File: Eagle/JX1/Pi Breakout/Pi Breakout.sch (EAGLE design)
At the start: 3 parts, among them J1 RASPBERRYPI-40-PIN-GPIO_PTH_N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, J2 RASPBERRYPI-40-PIN-GPIO_PTH_N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

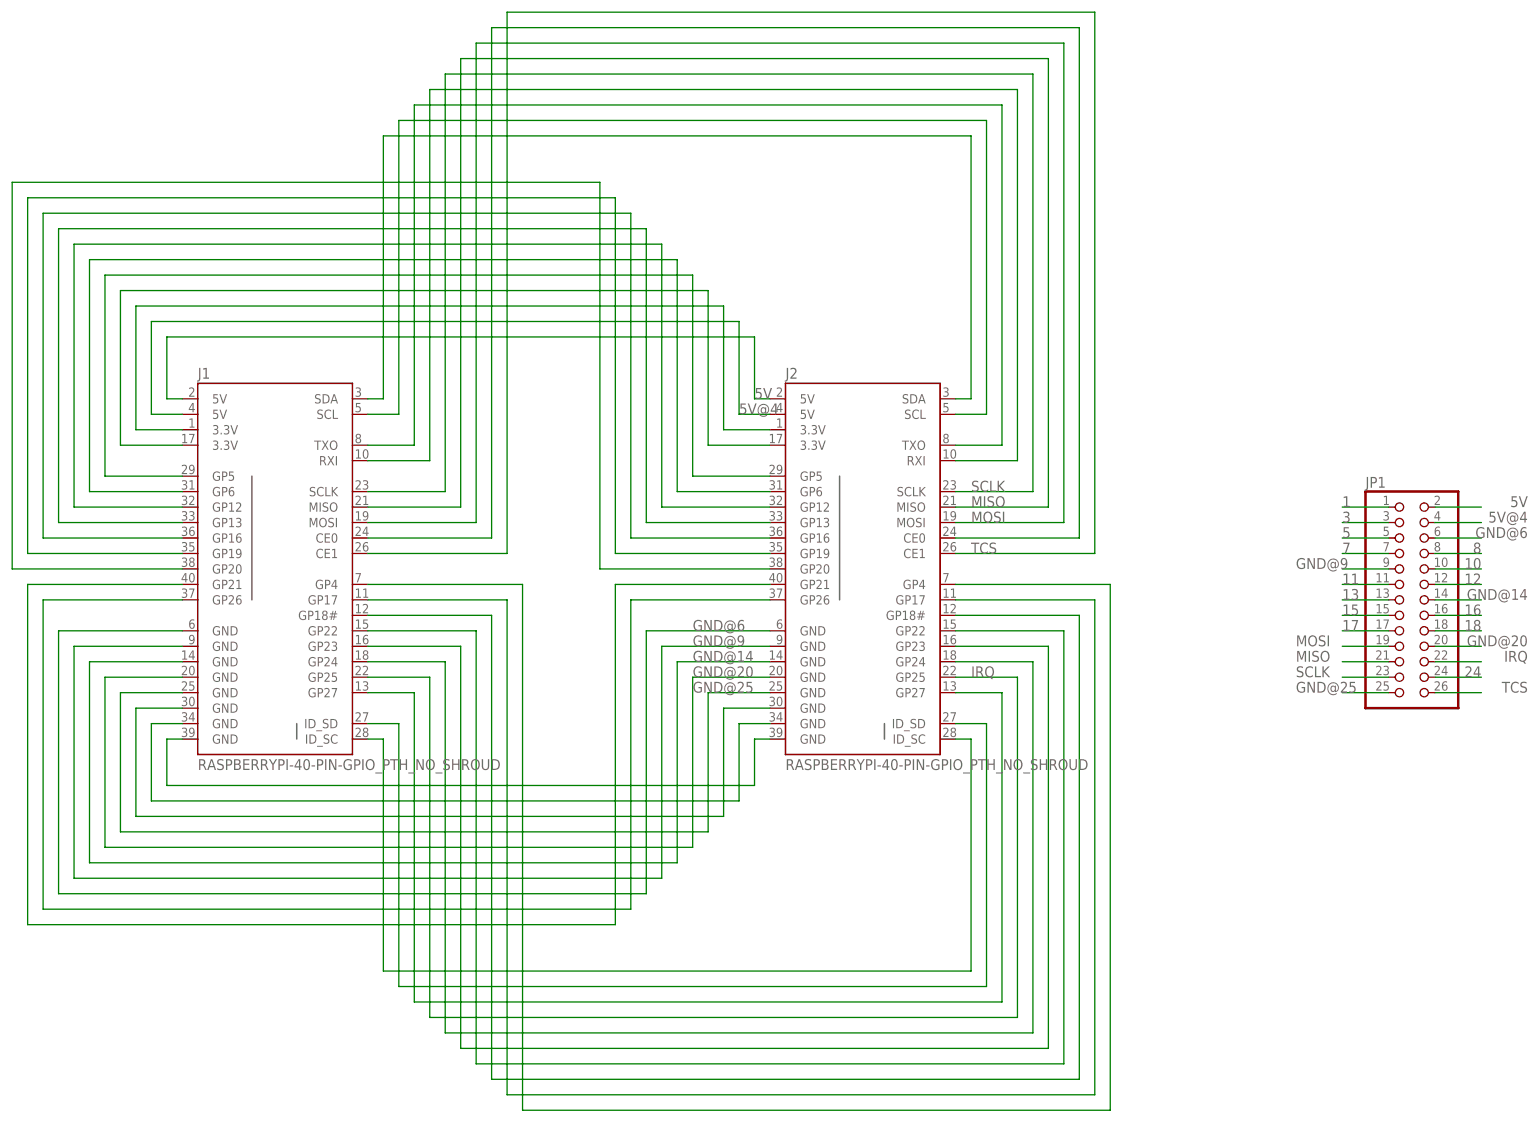
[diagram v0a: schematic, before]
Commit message: More board Changes
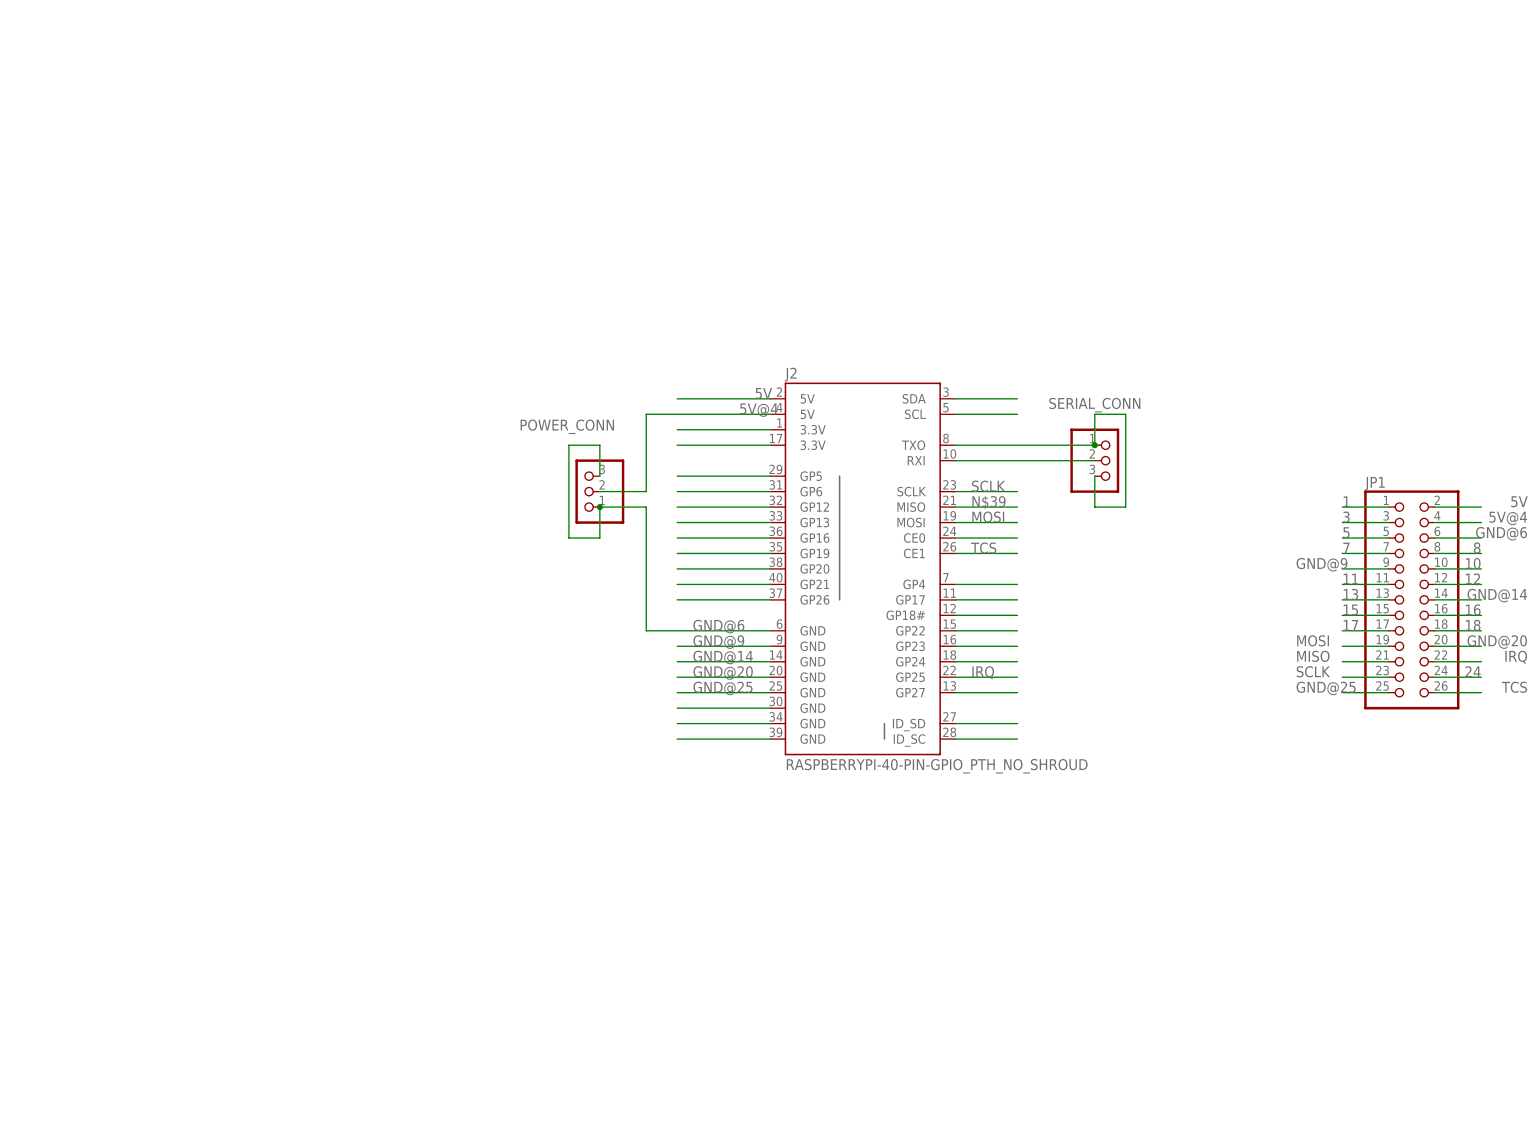
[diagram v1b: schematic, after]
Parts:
- removed J1: RASPBERRYPI-40-PIN-GPIO_PTH_NO_SHROUD, SparkFun-Connectors:RASPBERRYPI-40-PIN-GPIO_PTH_NO_SHROUD
- added POWER_CONN, SERIAL_CONN: (no value), pinhead:PINHD-1X3
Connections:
- removed net N$28: J1.SDA, J2.SDA
- removed net N$30: J1.RXI, J2.RXI
- removed net N$31: J1.TXO, J2.TXO
- removed net N$35: J1.CE0, J2.CE0
- new net N$1: J2.TXO, SERIAL_CONN.1, SERIAL_CONN.3
- new net N$25: J2.SDA
- new net N$32: J2.RXI, SERIAL_CONN.2
- new net N$33: J2.CE0
- new net N$39: J2.MISO
- net 5V: no longer J1.5V@2
- net 5V@4: now also POWER_CONN.2; no longer J1.5V@4
- net GND@14: no longer J1.GND@14
- net GND@20: no longer J1.GND@20
- net GND@25: no longer J1.GND@25
- net GND@6: now also POWER_CONN.1, POWER_CONN.3; no longer J1.GND@6
- net GND@9: no longer J1.GND@9
- net GP22: no longer J1.GP22
- net IRQ: no longer J1.GP25
- net MISO: no longer J1.MISO, J2.MISO
- net MOSI: no longer J1.MOSI
- net N$10: no longer J1.GND@30
- net N$16: no longer J1.GP26
- net N$17: no longer J1.GP13
- net N$18: no longer J1.GP16
- net N$19: no longer J1.GP21
- net N$20: no longer J1.GP19
- net N$21: no longer J1.GP20
- net N$22: no longer J1.ID_SC
- net N$23: no longer J1.ID_SD
- net N$24: no longer J1.GP27
- net N$26: no longer J1.GP24
- net N$27: no longer J1.GP23
- net N$29: no longer J1.SCL
- net N$3: no longer J1.3.3V@1
- net N$37: no longer J1.GP18#
- net N$38: no longer J1.GP17
- net N$4: no longer J1.3.3V@17
- net N$40: no longer J1.GP4
- net N$5: no longer J1.GP5
- net N$6: no longer J1.GP6
- net N$7: no longer J1.GP12
- net N$8: no longer J1.GND@39
- net N$9: no longer J1.GND@34
- net SCLK: no longer J1.SCLK
- net TCS: no longer J1.CE1
